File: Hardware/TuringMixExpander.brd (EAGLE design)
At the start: 105 x 50.3 mm, 46 parts, among them IC1 TL074P, IC2 TL072P

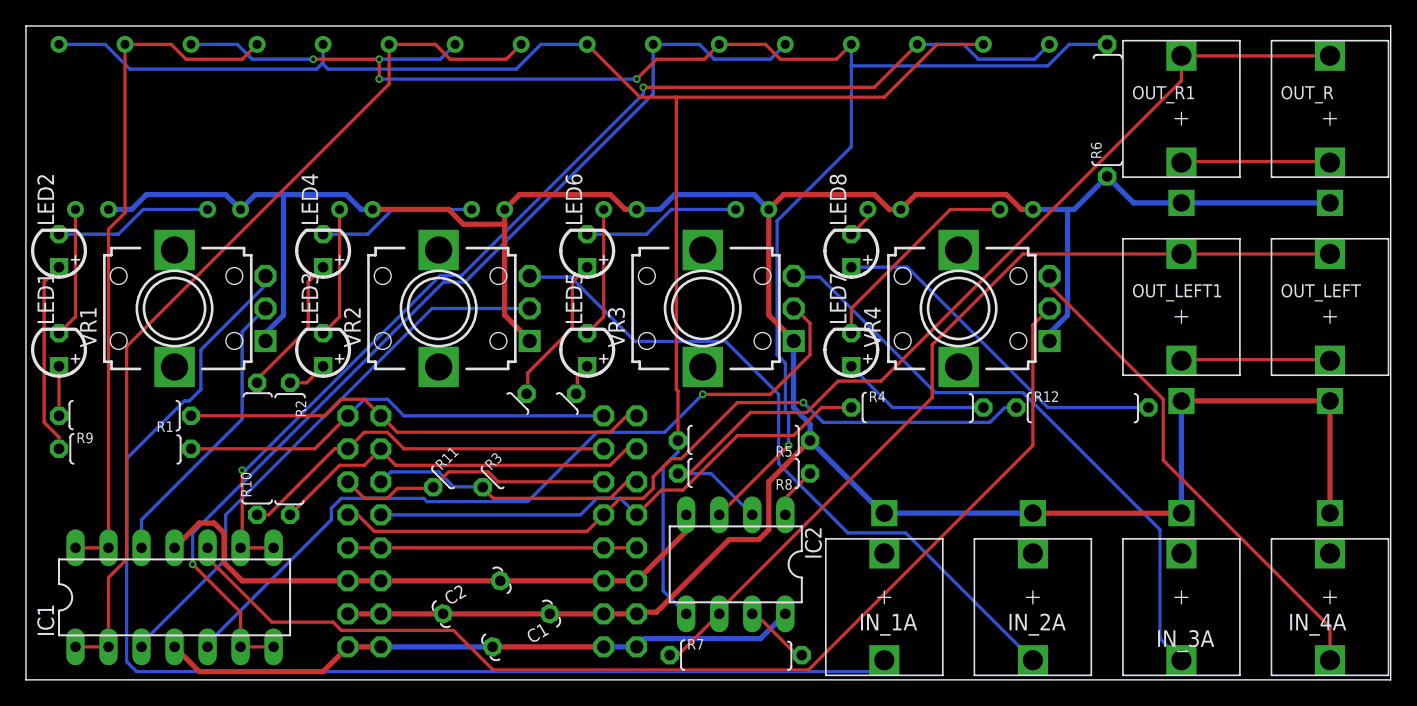
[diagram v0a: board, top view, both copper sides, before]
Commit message: New resistor grid
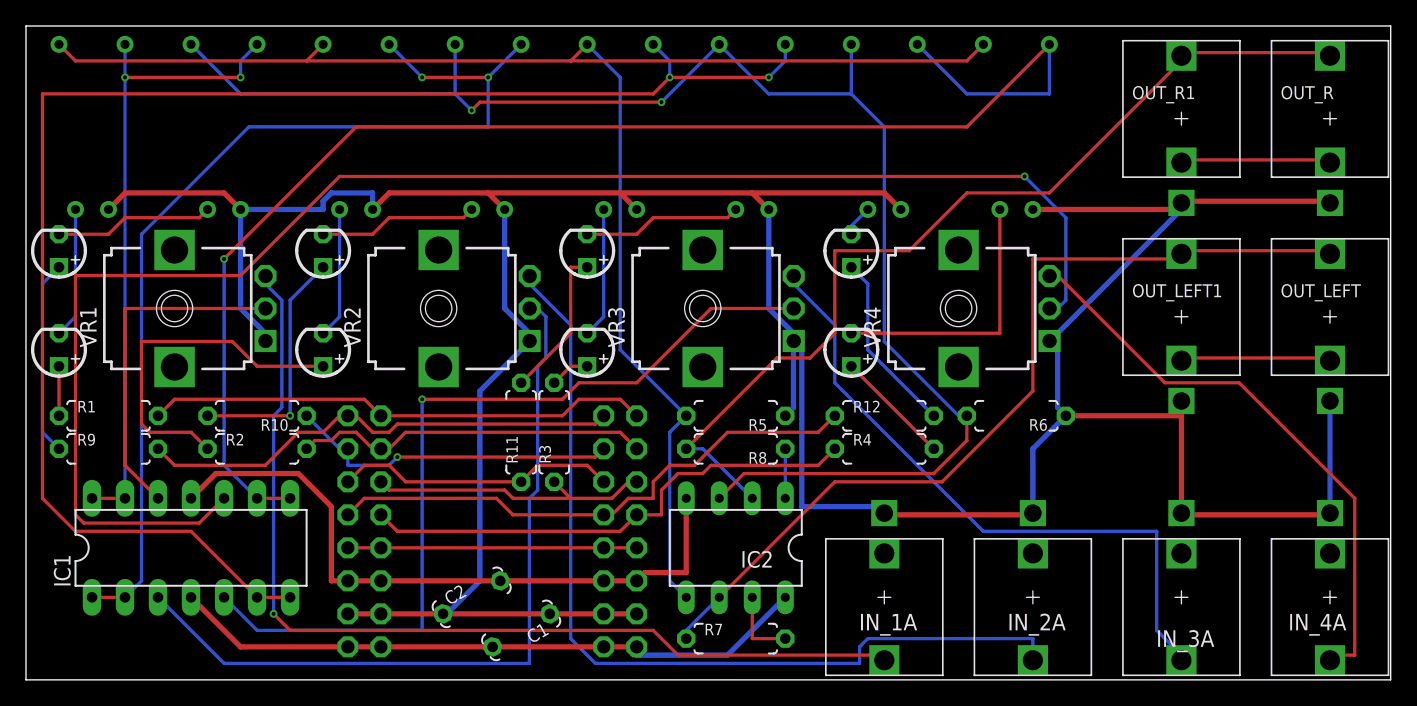
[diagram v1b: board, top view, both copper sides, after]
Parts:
- R1, R10, R11, R12, R2, R3, R4, R5, R6, R7, R8, R9: device TomW:0207/10 -> TomW:0207/7
- moved R6 24.5 mm to (76.2, 20.3), turned to 180 degrees
- moved R12 15.3 mm to (66.0, 20.3)
- moved R4 4.07 mm to (66.0, 17.8)
- moved IC1 4.02 mm to (12.7, 10.2)
- moved R11 3.24 mm to (38.1, 19.1), turned to 90 degrees
- moved R10 2.54 mm to (17.8, 20.3), turned to 180 degrees
- moved R2 2.54 mm to (17.8, 17.8), turned to 0 degrees
- moved R3 2.01 mm to (40.6, 19.1), turned to 90 degrees
- moved R5 2.01 mm to (54.6, 20.3)
- moved R8 2.01 mm to (54.6, 17.8)
- moved R1 1.27 mm to (6.35, 20.3), turned to 0 degrees
- moved R9 1.27 mm to (6.35, 17.8)
- moved R7 1.27 mm to (54.6, 3.17)
- moved IC2 1.27 mm to (54.6, 10.2)
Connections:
- net GATE1: now also R1.2; no longer R1.1
- net N$25: now also R1.1; no longer R1.2
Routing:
- net INPUT3: track 77.2 -> 115.9 mm, vias 1 -> 2
- net N$23: track 86.1 -> 119.4 mm, vias 0 -> 1
- net N$26: track 3.07 -> 27.0 mm
- net INPUT4: track 85.4 -> 107.9 mm, vias 2 -> 1
- net GND: track 257.5 -> 278.8 mm
- net N$1: track 93.4 -> 75.5 mm, vias 0 -> 1
- net N$4: track 42.8 -> 59.4 mm
- net GATE8: track 57.7 -> 42.4 mm, vias 1 -> 0
- net N$3: track 54.1 -> 68.8 mm
- net N$32: track 27.3 -> 14.1 mm
- net INPUT2: track 68.9 -> 77.2 mm, vias 0 -> 2
- net N$30: track 11.0 -> 18.8 mm, vias 0 -> 1
- net SUMR: track 122.7 -> 115.8 mm, vias 5 -> 2
- net N$13: track 38.5 -> 44.9 mm
- net -12V: track 46.2 -> 51.6 mm
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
